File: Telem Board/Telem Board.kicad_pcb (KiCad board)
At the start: 2 copper layers, 54 x 47.6 mm, 28 parts, among them J1 MAIN, J2 NTC1, J3 NTC2, J4 NTC3, J5 NTC4, J6 6S, J7 3S, U1 LM1117-3.3, U2 MCP3208

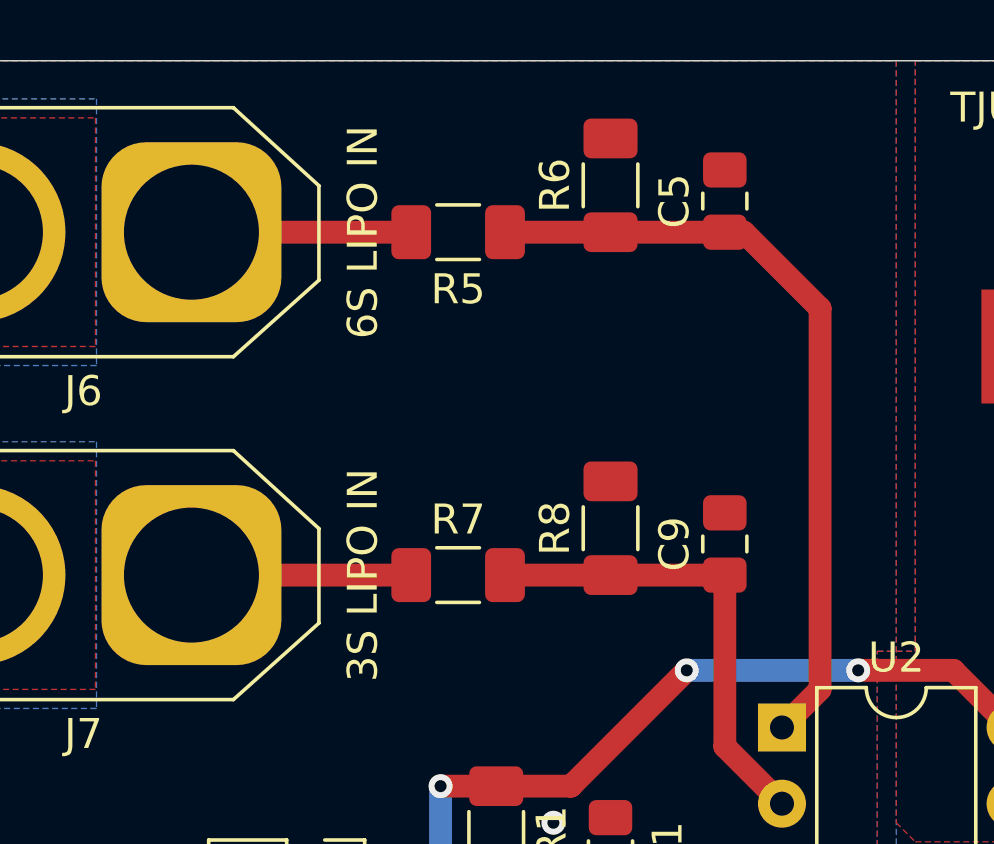
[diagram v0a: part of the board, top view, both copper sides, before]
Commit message: gerbers
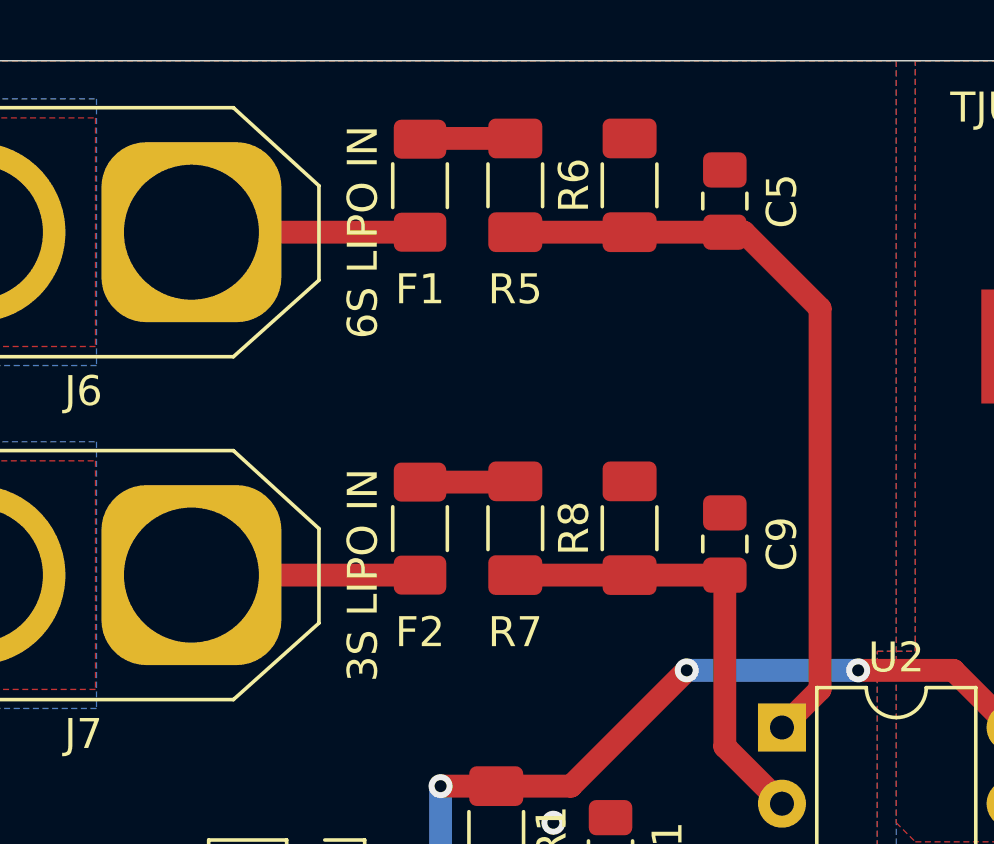
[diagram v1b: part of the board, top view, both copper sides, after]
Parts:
- added F1: 125mA, Resistor_SMD:R_1206_3216Metric_Pad1.30x1.75mm_HandSolder, F.Cu at (147.3, 68.3)
- added F2: 125mA, Resistor_SMD:R_1206_3216Metric_Pad1.30x1.75mm_HandSolder, F.Cu at (147.3, 79.7)
- moved R5 2.46 mm to (150.5, 68.3), turned to 270 degrees
- moved R7 2.46 mm to (150.5, 79.7), turned to 270 degrees
- moved R6 0.64 mm to (154.3, 68.3)
- moved R8 0.64 mm to (154.3, 79.7)
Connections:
- J6 pad 1: Net-(J6-Pad1) -> Net-(F1-Pad2)
- J7 pad 1: Net-(J7-Pad1) -> Net-(F2-Pad2)
- R5 pad 1: Net-(J6-Pad1) -> Net-(F1-Pad1)
- R7 pad 1: Net-(J7-Pad1) -> Net-(F2-Pad1)
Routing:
- net Net-(F2-Pad2): track 0.00 -> 7.62 mm
- net Net-(F1-Pad2): track 0.00 -> 7.62 mm
- net Net-(J7-Pad1): track 7.33 -> 0.00 mm
- net Net-(J6-Pad1): track 7.33 -> 0.00 mm
- net Net-(F2-Pad1): track 0.00 -> 3.19 mm
- net Net-(F1-Pad1): track 0.00 -> 3.19 mm
- removed copper zone on B.Cu, net (none)
- removed copper zone on F.Cu, net (none)
